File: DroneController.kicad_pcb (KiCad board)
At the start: 4 copper layers, 45.2 x 24.9 mm, 27 parts, among them P1 USB_C_Plug, U1 TP74333PDQNR, U3 BMP280, U4 MPU-6500, U6 L86-M33

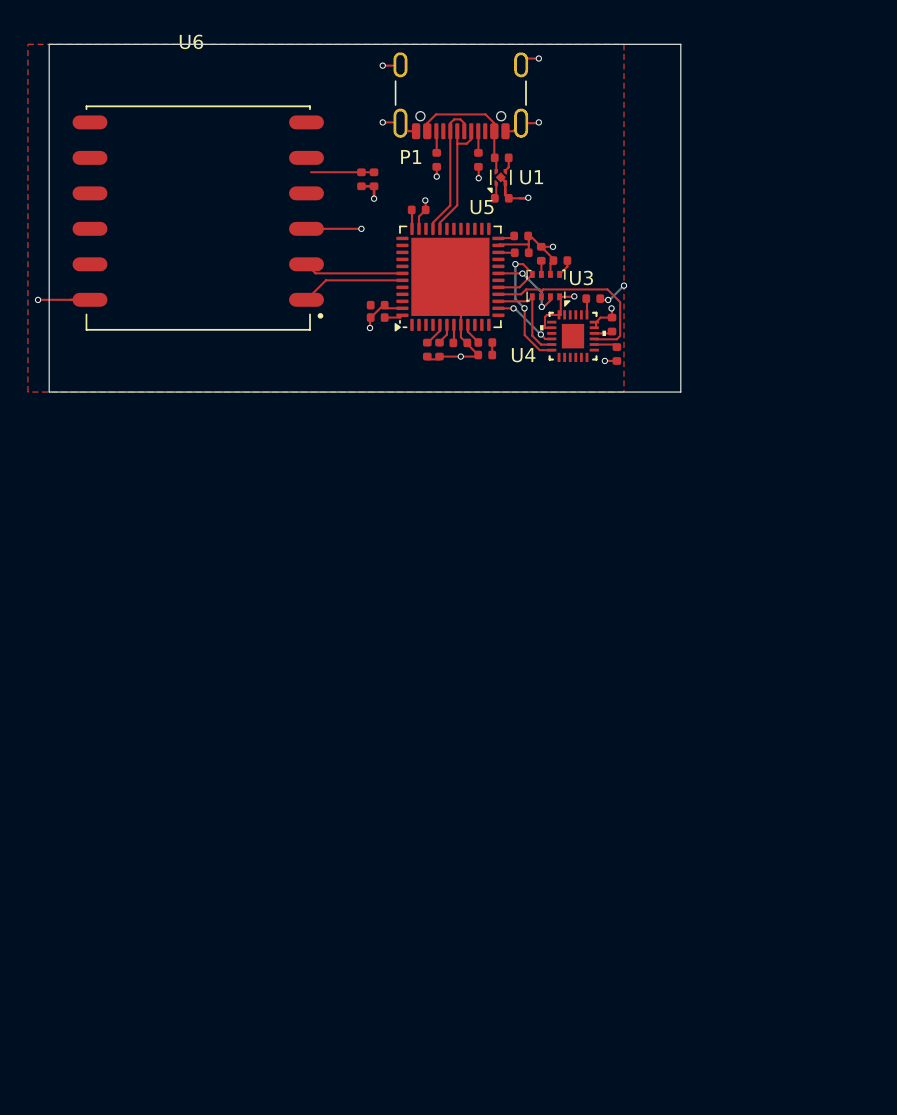
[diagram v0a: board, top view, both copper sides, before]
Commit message: Finalized PCB Design
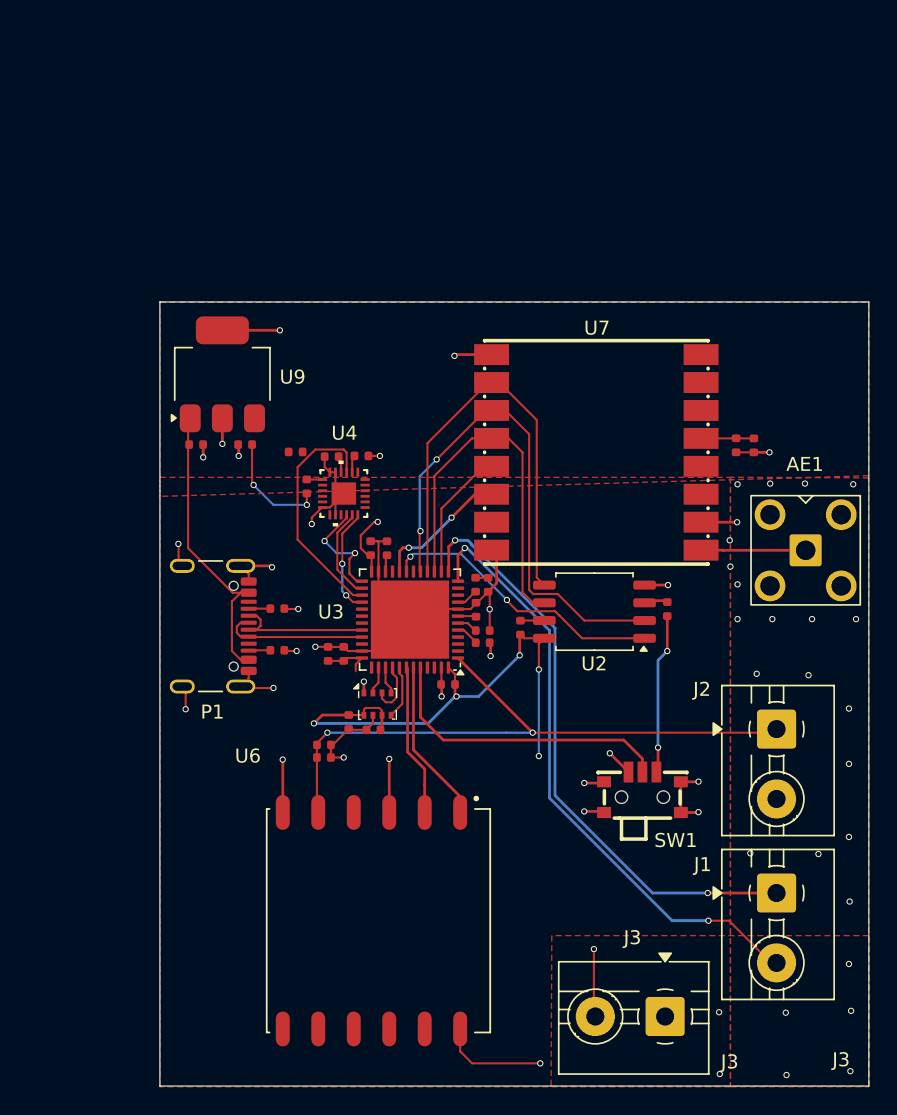
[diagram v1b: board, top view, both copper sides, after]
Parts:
- removed C14, C16: 1uF, PCM_JLCPCB:C_0402
- removed C4: 4.7uF, PCM_JLCPCB:C_0402
- removed U1: TP74333PDQNR, Package_DFN_QFN:OnSemi_XDFN4-1EP_1.0x1.0mm_EP0.52x0.52mm
- added AE1: 915MHZ Antenna, Connector_Coaxial:SMA_BAT_Wireless_BWSMA-KWE-Z001, F.Cu at (147.6, 122.6)
- added C28: 100nF, PCM_JLCPCB:C_0402, F.Cu at (143.9, 115.1)
- added C29: 100nF, PCM_JLCPCB:C_0402, F.Cu at (122.0, 132.2)
- added C5: 10uF, PCM_JLCPCB:C_0402, F.Cu at (142.6, 115.1)
- added C6: 10uF, PCM_JLCPCB:C_0402, F.Cu at (107.5, 115.0)
- added C8: 10uF, PCM_JLCPCB:C_0402, F.Cu at (104.0, 115.0)
- added J1: Connector, TerminalBlock:TerminalBlock_MaiXu_MX126-5.0-02P_1x02_P5.00mm, F.Cu at (145.5, 147.1)
- added J2: Connector, TerminalBlock:TerminalBlock_MaiXu_MX126-5.0-02P_1x02_P5.00mm, F.Cu at (145.5, 135.4)
- added J3: Connector, TerminalBlock:TerminalBlock_MaiXu_MX126-5.0-02P_1x02_P5.00mm, F.Cu at (137.6, 156.0)
- added R3: 5.1kΩ, PCM_JLCPCB:R_0402, F.Cu at (137.7, 126.8)
- added R4: 5.1kΩ, PCM_JLCPCB:R_0402, F.Cu at (127.2, 128.1)
- added R5: 5.1kΩ, PCM_JLCPCB:R_0402, F.Cu at (111.1, 115.5)
- added SW1: SW_SPDT, Switches:SW-SMD_MSK12CO2, F.Cu at (135.9, 139.9)
- added U2: W25Q16JVSS, Package_SO:SOIC-8_5.3x5.3mm_P1.27mm, F.Cu at (132.5, 127.0)
- added U7: 915MHz, Lora1276:COMM-SMD_LORA1276-C1-915MHZ, F.Cu at (132.6, 115.6)
- added U9: AP7361C-33E, Package_TO_SOT_SMD:SOT-223-3_TabPin2, F.Cu at (105.9, 110.0)
- moved U6 52.3 mm to (116.5, 149.1), turned to -90 degrees
- moved P1 43.4 mm to (104.1, 128.0), turned to -90 degrees
- moved C15 41.5 mm to (113.1, 137.4), turned to 0 degrees
- moved C31 40.7 mm to (113.1, 136.5), turned to 0 degrees
- moved R2 36.9 mm to (109.8, 129.7), turned to 180 degrees
- moved C12 36.3 mm to (114.9, 134.9), turned to -90 degrees
- moved C17 36.1 mm to (116.7, 135.4), turned to 180 degrees
- moved R1 35.2 mm to (109.8, 126.8), turned to 180 degrees
- moved U3 32.3 mm to (117.0, 133.6), turned to 0 degrees
- moved C25 25.1 mm to (114.6, 130.0), turned to -90 degrees
- moved C9 24.8 mm to (116.5, 122.4), turned to -90 degrees
- moved U5 24.7 mm to (119.3, 127.5), turned to 180 degrees
- moved C3 24.5 mm to (111.9, 118.0), turned to 90 degrees
- moved C18 24.3 mm to (113.4, 130.0), turned to 90 degrees
- moved C26 23.3 mm to (117.7, 122.4), turned to 90 degrees
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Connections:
- U3 pad 2: /SPI5_NSS -> /SPI3_NSS
- U3 pad 3: /SPI1_MISO -> /SPI3_MISO
- U3 pad 4: /SPI1_SCK -> /SPI3_SCK
- U3 pad 5: /SPI1_MOSI -> /SPI3_MOSI
- U4 pad 22: /SPI1_NSS -> /SPI2_NSS
- U4 pad 23: /SPI1_SCK -> /SPI2_SCK
- U4 pad 24: /SPI1_MOSI -> /SPI2_MOSI
- U4 pad 25: unconnected-(U4-Pad25) -> GND
- U4 pad 9: /SPI1_MISO -> /SPI2_MISO
- U5 pad 12: unconnected-(U5-PA2-Pad12) -> /USART2_TX
- U5 pad 13: unconnected-(U5-PA3-Pad13) -> /USART2_RX
- U5 pad 18: unconnected-(U5-PB0-Pad18) -> /SPI5_SCK
- U5 pad 20: unconnected-(U5-PB2-Pad20) -> /Lora_RES
- U5 pad 25: unconnected-(U5-PB12-Pad25) -> /SPI2_NSS
- U5 pad 26: unconnected-(U5-PB13-Pad26) -> /SPI2_SCK
- U5 pad 27: unconnected-(U5-PB14-Pad27) -> /SPI2_MISO
- U5 pad 28: unconnected-(U5-PB15-Pad28) -> /SPI2_MOSI
- U5 pad 38: unconnected-(U5-PA15-Pad38) -> /SPI3_NSS
- U5 pad 39: unconnected-(U5-PB3-Pad39) -> /SPI3_SCK
- U5 pad 40: unconnected-(U5-PB4-Pad40) -> /SPI3_MISO
- U5 pad 41: unconnected-(U5-PB5-Pad41) -> /SPI3_MOSI
- U5 pad 44: unconnected-(U5-BOOT0-Pad44) -> Net-(SW1-B)
- U6 pad 6: unconnected-(U6-1PPS-Pad6) -> GND
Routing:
- net +3.3V: track 11.3 -> 71.6 mm, vias 2 -> 10
- net GND: track 56.0 -> 106.7 mm, vias 17 -> 57
- net /USART2_TX: track 0.00 -> 44.2 mm, vias 0 -> 2
- net /USART2_RX: track 0.00 -> 43.0 mm, vias 0 -> 2
- net +BATT: track 4.18 -> 45.2 mm, vias 0 -> 2
- net /SPI1_MOSI: track 12.2 -> 37.7 mm
- net Net-(SW1-B): track 0.00 -> 21.6 mm
- net /SPI1_SCK: track 7.13 -> 26.6 mm
- net /SPI1_MISO: track 14.0 -> 32.0 mm
- net /SPI2_MISO: track 0.00 -> 17.0 mm
- net /SPI5_NSS: track 5.76 -> 20.6 mm
- net +5V: track 9.35 -> 21.6 mm
- net /Lora_RES: track 0.00 -> 9.73 mm, vias 0 -> 2
- net /SPI2_NSS: track 0.00 -> 7.84 mm, vias 0 -> 2
- net /SPI2_MOSI: track 0.00 -> 7.67 mm, vias 0 -> 2
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- added copper zone on F.Cu, net GND
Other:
- board size 45.2 x 24.9 mm -> 50.7 x 56.1 mm
- board text added: "Flight Controller"
- board text added: "J3"
